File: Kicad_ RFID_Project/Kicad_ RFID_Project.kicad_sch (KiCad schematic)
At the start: 18 parts, among them J1 Conn_01x08, J2 Conn_ST_STDC14, J3 USB_C_Receptacle_USB2.0_14P, SW1 RESET, U1 STM32L476RGTx, U2 AZ1117CH2-3.3

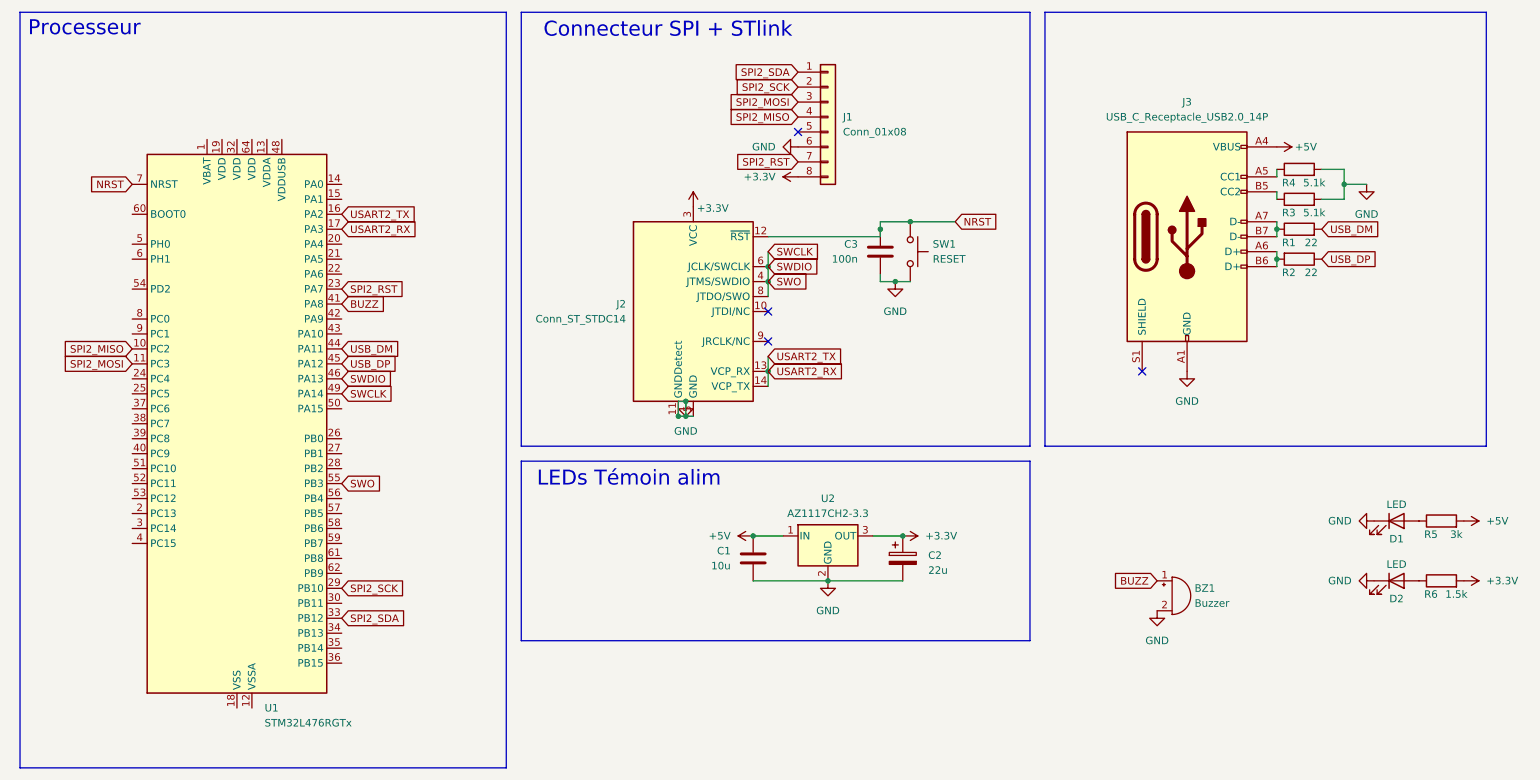
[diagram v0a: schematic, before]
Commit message: changement kicad
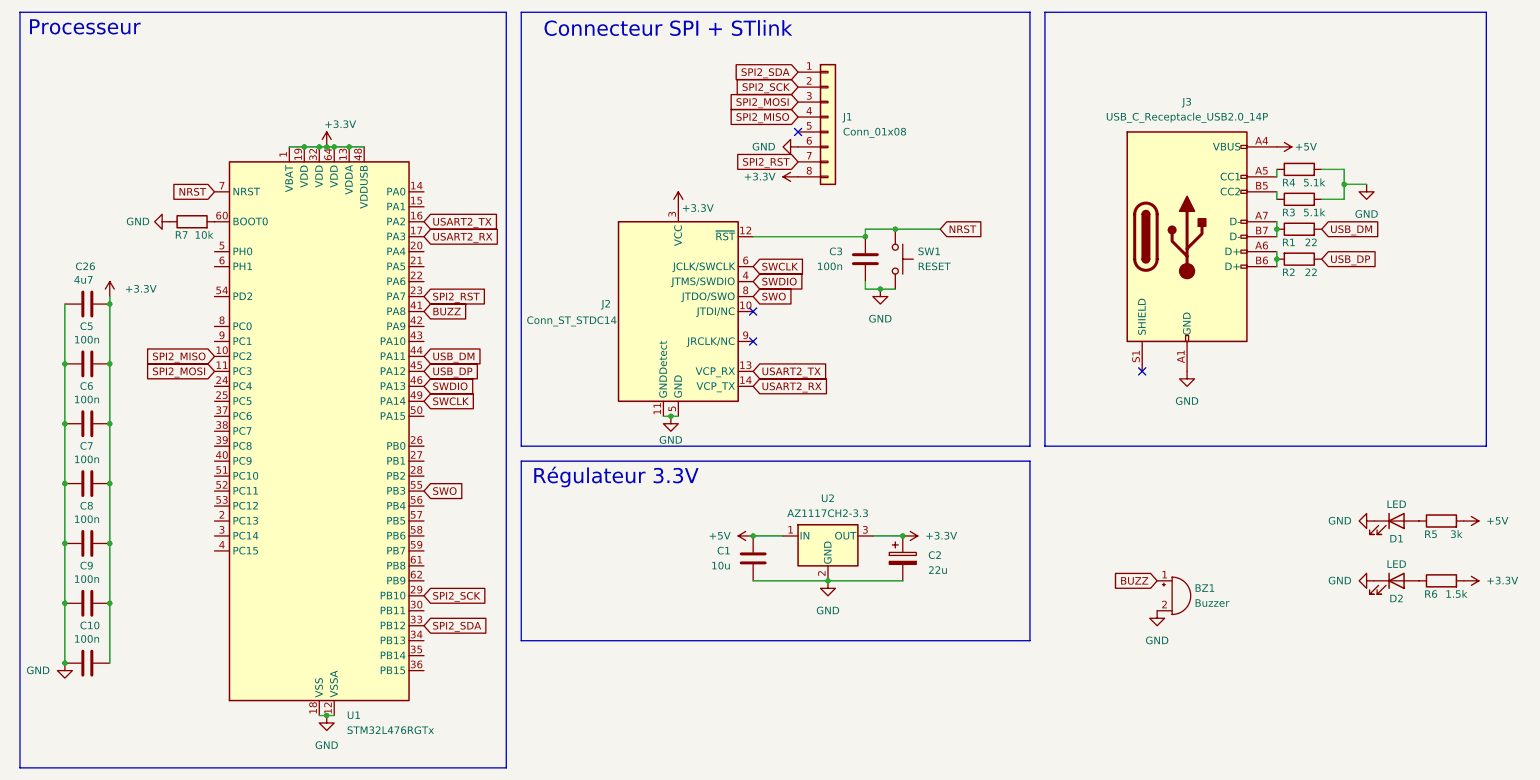
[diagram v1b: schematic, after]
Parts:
- added C10, C5, C6, C7, C8, C9: 100n, Capacitor_SMD:C_0402_1005Metric, symbol Device:C
- added C26: 4u7, Capacitor_SMD:C_0402_1005Metric, symbol Device:C
- added R7: 10k, symbol Device:R
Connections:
- net +3.3V: now also U1.1 (VBAT), U1.13 (VDDA), U1.19 (VDD), U1.32 (VDD), U1.48 (VDDUSB), U1.64 (VDD), C10.2, C26.2, C5.2, C6.2, C7.2, C8.2, C9.2
- net GND: now also U1.12 (VSSA), U1.18 (VSS), U1.31 (VSS), U1.47 (VSS), U1.63 (VSS), C10.1, C26.1, C5.1, C6.1, C7.1, C8.1, C9.1, R7.1
- net SWCLK: no longer J2.4 (JTMS/SWDIO), J2.8 (JTDO/SWO), U1.46 (PA13), U1.55 (PB3)
- net USART2_RX: no longer J2.13 (VCP_RX), U1.16 (PA2)
- net at U1.60 (BOOT0): now also R7.2
- new net SWDIO: J2.4 (JTMS/SWDIO), U1.46 (PA13)
- new net SWO: J2.8 (JTDO/SWO), U1.55 (PB3)
- new net USART2_TX: J2.13 (VCP_RX), U1.16 (PA2)
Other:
- note added: "Régulateur 3.3V"
- note removed: "LEDs Témoin alim"
- moved on the sheet: C3, J2, SW1, U1
